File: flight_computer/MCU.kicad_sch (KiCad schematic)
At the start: 37 parts, among them J1 Conn_02x05_Odd_Even, J2 MEM2061-01-188-00-A_REVA, Q1 Q_NPN_BEC, SW1 SW_Push, SW2 SW_Push, U2 STM8S007C8T6TR, Y1 12MHz

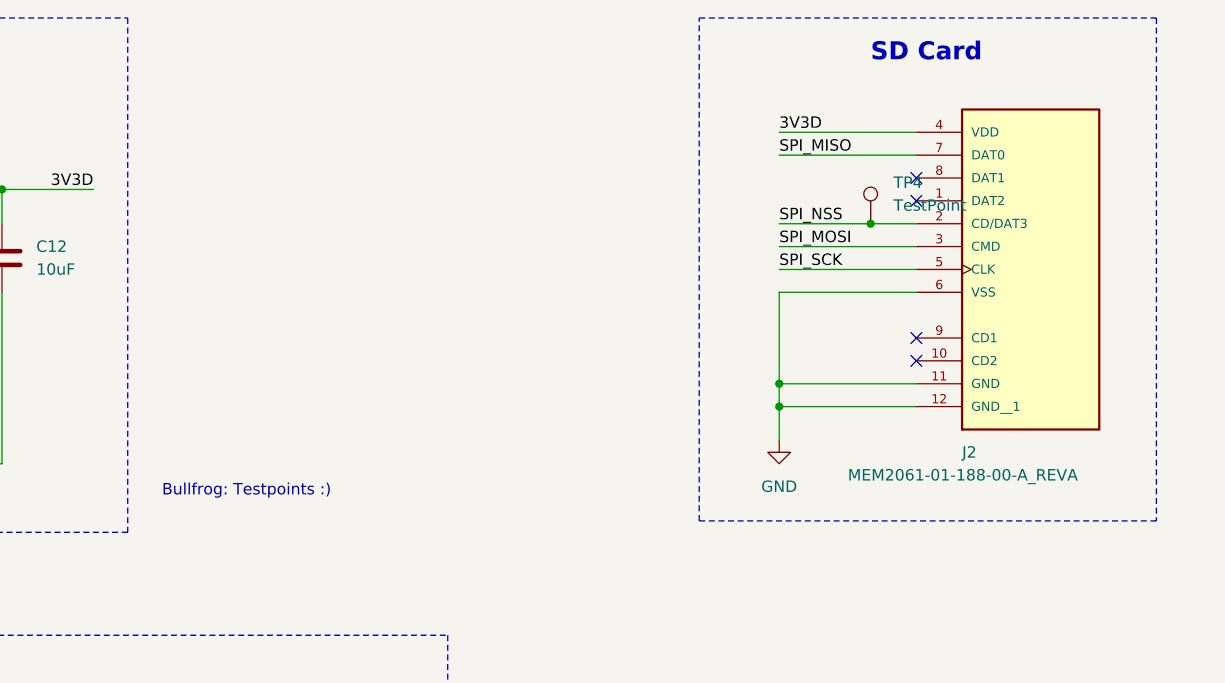
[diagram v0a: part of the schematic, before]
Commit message: Most of the way through relayout and new antenna
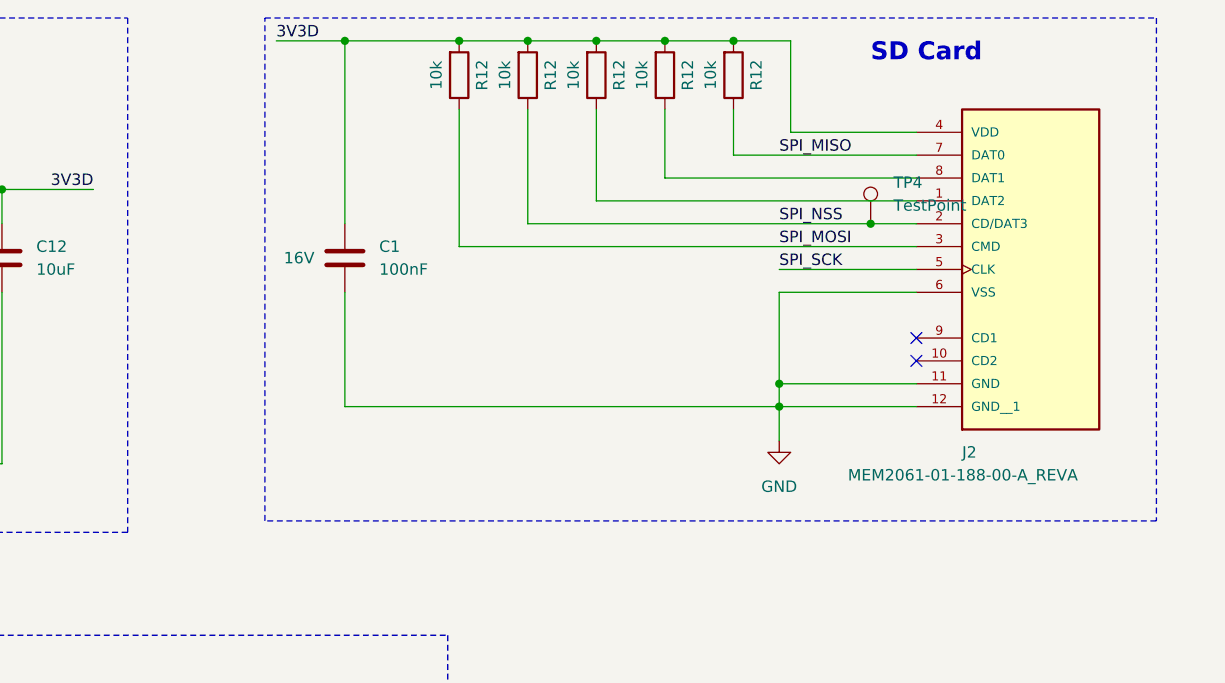
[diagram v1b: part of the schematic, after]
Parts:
- added C1: 100nF, Capacitor_SMD:C_0402_1005Metric, symbol Device:C
- added R12 (x5): 10k, Resistor_SMD:R_0402_1005Metric, symbol Device:R
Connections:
- net 3V3D: now also C1.1, R12.2, R12.2, R12.2, R12.2, R12.2
- net GND: now also C1.2
- net SPI_MISO: now also R12.1
- net SPI_MOSI: now also R12.1
- net SPI_NSS: now also R12.1
- net at J2.1 (DAT2): now also R12.1
- net at J2.8 (DAT1): now also R12.1
- no-connect marks 21 -> 19
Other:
- note removed: "Bullfrog: Testpoints :)"
